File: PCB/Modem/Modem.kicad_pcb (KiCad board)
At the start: 6 copper layers, 64.6 x 58.9 mm, 211 parts, among them IC10 AT32 433, IC11 29F040A-12 (I-Reverse, IC12 KM681000BLT-7 (I-Reverse), IC13 EA, IC14 E4, IC15 8206 5877, IC16 E3, IC17 EA, IC18 3L01, IC2 EA, IC3 Line-Module, IC4 E5, IC5 MN195, IC6 54, IC7 EA, IC8 TA31033F, IC9 EA, Q1 CQ, Q2 DA QU, Q3 123, Q4 CQ, Q7 SOT-323_SC-70, Q9 HP, SW2 SW_modem, T1 IsoTransformer

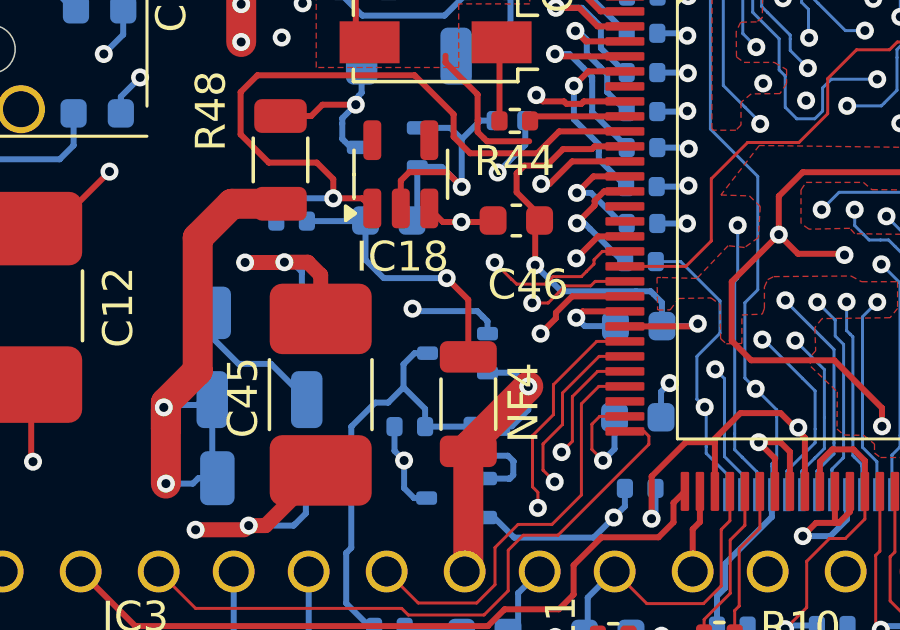
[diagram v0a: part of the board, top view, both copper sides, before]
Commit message: Add files via upload
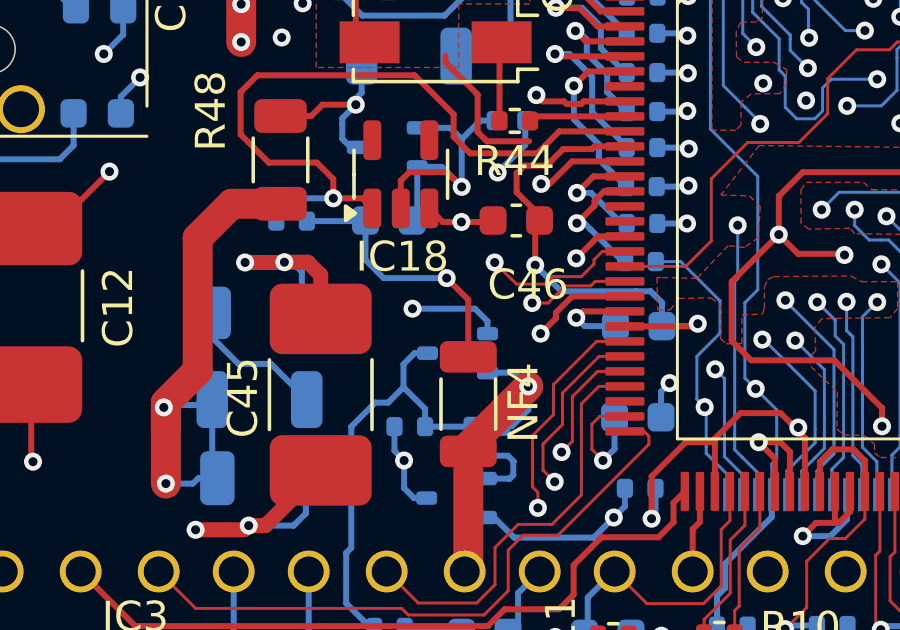
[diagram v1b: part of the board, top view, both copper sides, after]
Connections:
- net J13_58_PC110 renamed MN192_S11_BUF
- net PNET5_Q31_PC110 renamed Pluto_Enabled_PNET5
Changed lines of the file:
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@@
 	(net 1 "PNET1")
 	(net 2 "VCC_PC110")
-	(net 3 "PNET5_Q31_PC110")
+	(net 3 "Pluto_Enabled_PNET5")
 	(net 4 "PNET4")
 	(net 5 "GND")
@@
 	(net 40 "J13_42_PC110")
 	(net 41 "J13_41_PC110")
-	(net 42 "J13_58_PC110")
+	(net 42 "MN192_S11_BUF")
 	(net 43 "MN195_IRQ1#")
 	(net 44 "MN195_VPCK#")
@@
 			(layers "F.Cu" "F.Mask" "F.Paste")
 			(roundrect_rratio 0.25)
-			(net 3 "PNET5_Q31_PC110")
+			(net 3 "Pluto_Enabled_PNET5")
 		)
 		(embedded_fonts no)
@@
 			(size 1.6 1.1)
 			(layers "F.Cu" "F.Mask" "F.Paste")
-			(net 3 "PNET5_Q31_PC110")
+			(net 3 "Pluto_Enabled_PNET5")
 			(thermal_bridge_angle 45)
 		)
@@
 			(layers "F.Cu" "F.Mask" "F.Paste")
 			(roundrect_rratio 0.25)
-			(net 3 "PNET5_Q31_PC110")
+			(net 3 "Pluto_Enabled_PNET5")
 		)
 		(embedded_fonts no)
@@
 			(size 2.286 0.65)
 			(layers "F.Cu" "F.Mask" "F.Paste")
-			(net 3 "PNET5_Q31_PC110")
+			(net 3 "Pluto_Enabled_PNET5")
 			(thermal_bridge_angle 45)
 		)
@@
 			(size 2.286 0.65)
 			(layers "F.Cu" "F.Mask" "F.Paste")
-			(net 3 "PNET5_Q31_PC110")
+			(net 3 "Pluto_Enabled_PNET5")
 			(thermal_bridge_angle 45)
 		)
@@
 			(size 2.286 0.65)
 			(layers "F.Cu" "F.Mask" "F.Paste")
-			(net 42 "J13_58_PC110")
+			(net 42 "MN192_S11_BUF")
 			(thermal_bridge_angle 45)
 		)
@@
 			(layers "F.Cu" "F.Mask" "F.Paste")
 			(roundrect_rratio 0.25)
-			(net 3 "PNET5_Q31_PC110")
+			(net 3 "Pluto_Enabled_PNET5")
 		)
 		(embedded_fonts no)
@@
 			(layers "F.Cu" "F.Mask" "F.Paste")
 			(roundrect_rratio 0.2)
-			(net 3 "PNET5_Q31_PC110")
+			(net 3 "Pluto_Enabled_PNET5")
 		)
 		(pad "3" smd roundrect
@@
 			(layers "B.Cu" "B.Mask" "B.Paste")
 			(roundrect_rratio 0.217391)
-			(net 3 "PNET5_Q31_PC110")
+			(net 3 "Pluto_Enabled_PNET5")
 		)
 		(embedded_fonts no)
@@
 			(layers "B.Cu" "B.Mask" "B.Paste")
 			(roundrect_rratio 0.25)
-			(net 3 "PNET5_Q31_PC110")
+			(net 3 "Pluto_Enabled_PNET5")
 		)
 		(embedded_fonts no)
@@
 			(layers "B.Cu" "B.Mask" "B.Paste")
 			(roundrect_rratio 0.25)
-			(net 3 "PNET5_Q31_PC110")
+			(net 3 "Pluto_Enabled_PNET5")
 		)
 		(embedded_fonts no)
@@
 			(layers "B.Cu" "B.Mask" "B.Paste")
 			(roundrect_rratio 0.25)
-			(net 42 "J13_58_PC110")
+			(net 42 "MN192_S11_BUF")
 		)
 		(pad "3" smd roundrect
@@
 			(layers "B.Cu" "B.Mask" "B.Paste")
 			(roundrect_rratio 0.25)
-			(net 3 "PNET5_Q31_PC110")
+			(net 3 "Pluto_Enabled_PNET5")
 		)
 		(pad "2" smd roundrect
@@
 			(layers "B.Cu" "B.Mask" "B.Paste")
 			(roundrect_rratio 0.25)
-			(net 3 "PNET5_Q31_PC110")
+			(net 3 "Pluto_Enabled_PNET5")
 		)
 		(embedded_fonts no)
@@
 			(layers "B.Cu" "B.Mask" "B.Paste")
 			(roundrect_rratio 0.25)
-			(net 42 "J13_58_PC110")
+			(net 42 "MN192_S11_BUF")
 		)
 		(embedded_fonts no)
@@
 	)
 	(segment
-		(start 136.41 115.1)
-		(end 136.33 115.02)
-		(width 0.2)
-		(layer "B.Cu")
-		(net 78)
-	)
-	(segment
 		(start 138.83 115.8525)
 		(end 138.83 115.44)
@@
 	)
 	(segment
-		(start 138.14 115.1)
-		(end 136.41 115.1)
-		(width 0.2)
-		(layer "B.Cu")
-		(net 78)
-	)
-	(segment
-		(start 138.49 115.1)
-		(end 138.14 115.1)
+		(start 138.41 115.02)
+		(end 136.33 115.02)
 		(width 0.2)
 		(layer "B.Cu")
@@
 	(segment
 		(start 138.83 115.44)
-		(end 138.67 115.28)
-		(width 0.2)
-		(layer "B.Cu")
-		(net 78)
-	)
-	(segment
-		(start 138.67 115.28)
-		(end 138.49 115.1)
+		(end 138.41 115.02)
 		(width 0.2)
 		(layer "B.Cu")
@@
 	(zone
 		(net 3)
-		(net_name "PNET5_Q31_PC110")
+		(net_name "Pluto_Enabled_PNET5")
 		(layer "In3.Cu")
 		(hatch edge 0.5)

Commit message: Add files via upload
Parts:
- IC11: value 29F040A-12 (I-Reverse -> EN29F040A
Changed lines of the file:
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@@
 			)
 		)
-		(property "Value" "29F040A-12 (I-Reverse"
+		(property "Value" "EN29F040A"
 			(at 0 -11.3 0)
 			(layer "B.Fab")
